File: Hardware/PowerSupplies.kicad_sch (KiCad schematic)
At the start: 56 parts

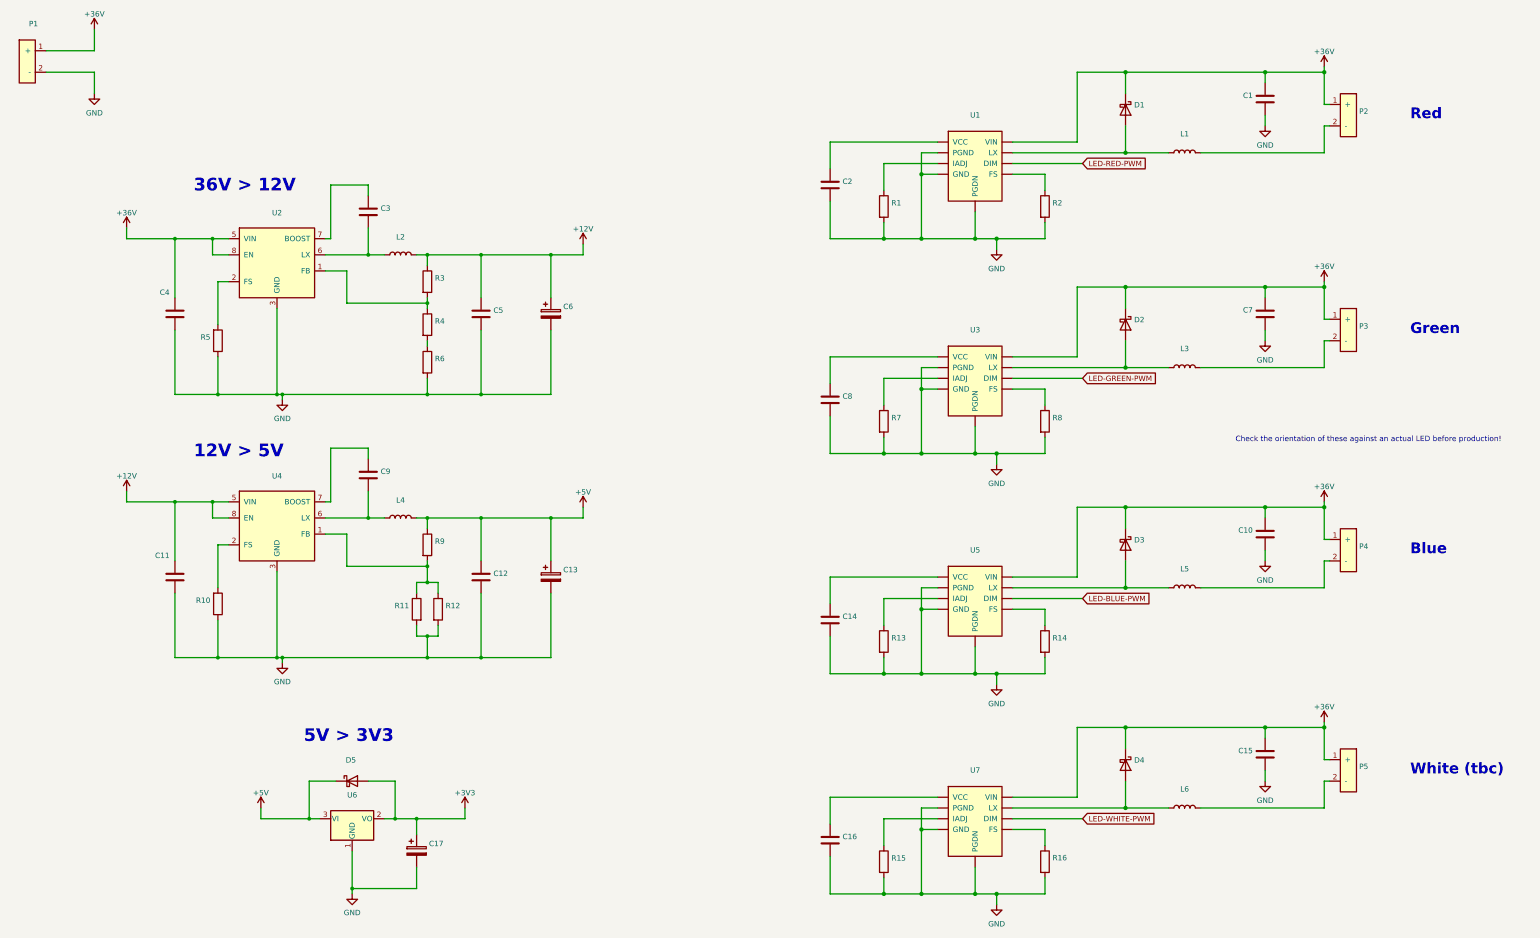
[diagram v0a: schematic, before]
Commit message: Xtal footprint selected. Remaining parts need new footprints.
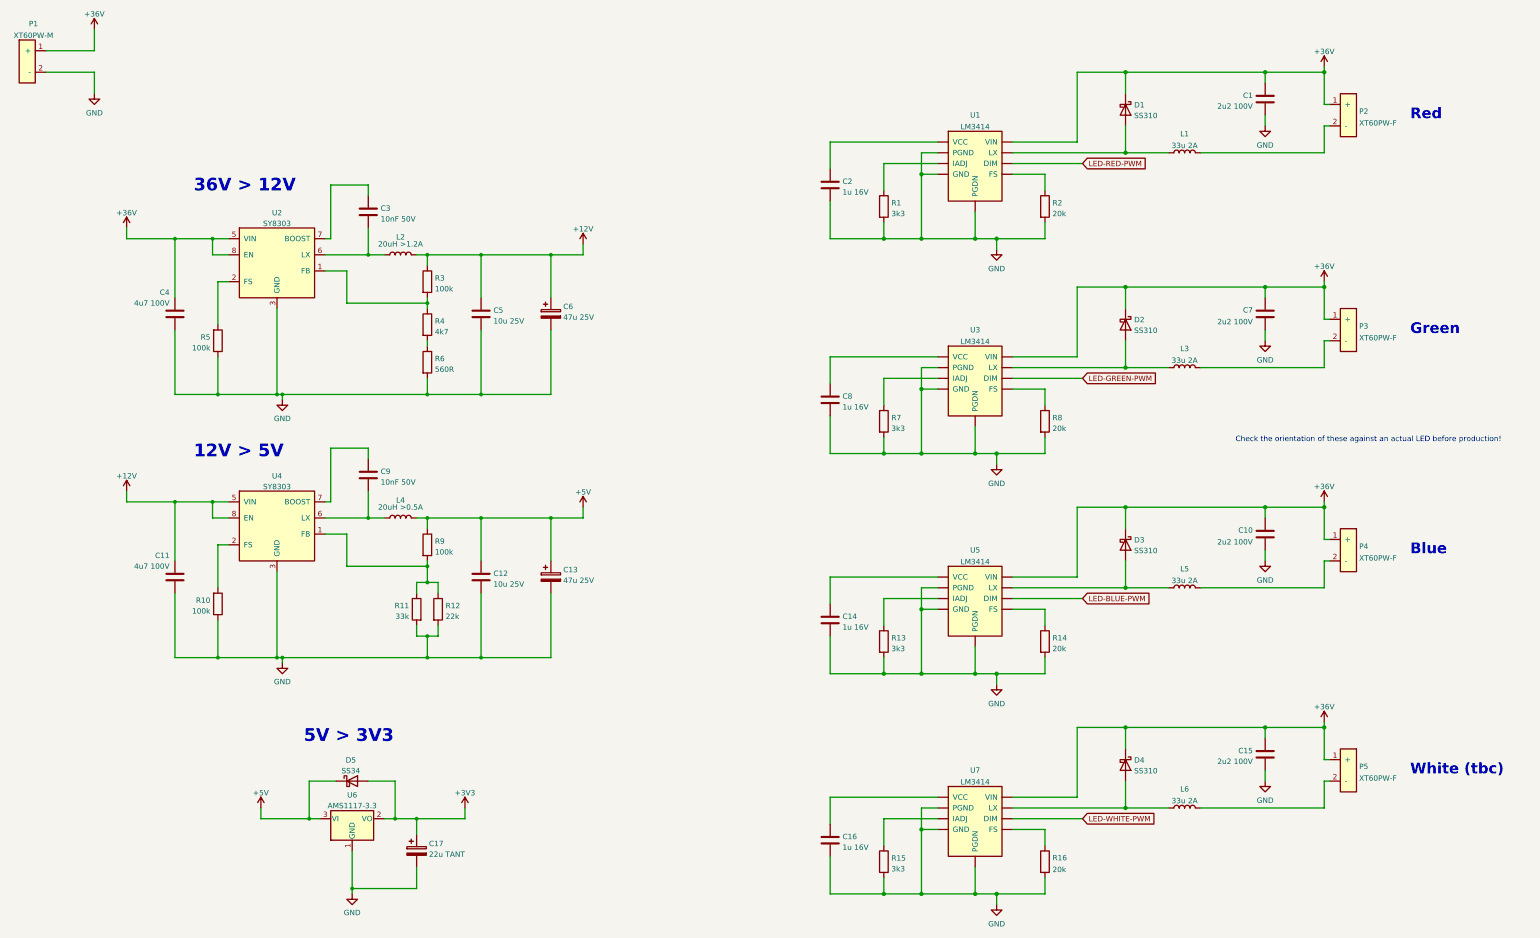
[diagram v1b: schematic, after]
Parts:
- C1, C10, C15, C7: value (none) -> 2u2 100V; footprint (none) -> Capacitor_SMD:CP_Elec_6.3x5.4
- C11, C4: value (none) -> 4u7 100V; footprint (none) -> Capacitor_SMD:C_1210_3225Metric
- C12, C5: value (none) -> 10u 25V; footprint (none) -> Capacitor_SMD:C_0805_2012Metric_Pad1.18x1.45mm_HandSolder
- C13, C6: value (none) -> 47u 25V; footprint (none) -> Capacitor_SMD:CP_Elec_6.3x5.4
- C14, C16, C2, C8: value (none) -> 1u 16V; footprint (none) -> Capacitor_SMD:C_0805_2012Metric_Pad1.18x1.45mm_HandSolder
- C17: value (none) -> 22u TANT; footprint (none) -> Capacitor_Tantalum_SMD:CP_EIA-3528-15_AVX-H
- C3, C9: value (none) -> 10nF 50V; footprint (none) -> Capacitor_SMD:C_0805_2012Metric_Pad1.18x1.45mm_HandSolder
- D1, D2, D3, D4: value (none) -> SS310; footprint (none) -> Diode_SMD:D_SMA_Handsoldering
- D5: value (none) -> SS34; footprint (none) -> Diode_SMD:D_SMA_Handsoldering
- L1, L3, L5, L6: value (none) -> 33u 2A; footprint (none) -> Inductor_SMD:L_SigTra_SC3316F
- L2: value (none) -> 20uH >1.2A; footprint (none) -> Inductor_SMD:L_Taiyo-Yuden_NR-80xx
- L4: value (none) -> 20uH >0.5A; footprint (none) -> Inductor_SMD:L_Taiyo-Yuden_NR-80xx
- P1: value (none) -> XT60PW-M; footprint (none) -> PersonalConnectors:AMASS_XT60PW-M
- P2, P3, P4, P5: value (none) -> XT60PW-F; footprint (none) -> PersonalConnectors:AMASS_XT60PW-F
- R1, R13, R15, R7: value (none) -> 3k3; footprint (none) -> Resistor_SMD:R_0603_1608Metric_Pad0.98x0.95mm_HandSolder
- R10, R3, R5, R9: value (none) -> 100k; footprint (none) -> Resistor_SMD:R_0603_1608Metric_Pad0.98x0.95mm_HandSolder
- R11: value (none) -> 33k; footprint (none) -> Resistor_SMD:R_0603_1608Metric_Pad0.98x0.95mm_HandSolder
- R12: value (none) -> 22k; footprint (none) -> Resistor_SMD:R_0603_1608Metric_Pad0.98x0.95mm_HandSolder
- R14, R16, R2, R8: value (none) -> 20k; footprint (none) -> Resistor_SMD:R_0603_1608Metric_Pad0.98x0.95mm_HandSolder
- R4: value (none) -> 4k7; footprint (none) -> Resistor_SMD:R_0603_1608Metric_Pad0.98x0.95mm_HandSolder
- R6: value (none) -> 560R; footprint (none) -> Resistor_SMD:R_0603_1608Metric_Pad0.98x0.95mm_HandSolder
- U1, U3, U5, U7: value (none) -> LM3414; footprint (none) -> PersonalDiscretes:TI_SO-PowerPAD-8_HandSolder
- U2, U4: value (none) -> SY8303; footprint (none) -> Package_TO_SOT_SMD:TSOT-23-8
- U6: value (none) -> AMS1117-3.3; footprint (none) -> Package_TO_SOT_SMD:SOT-223-3_TabPin2

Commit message: USB footprint added, mount holes added.
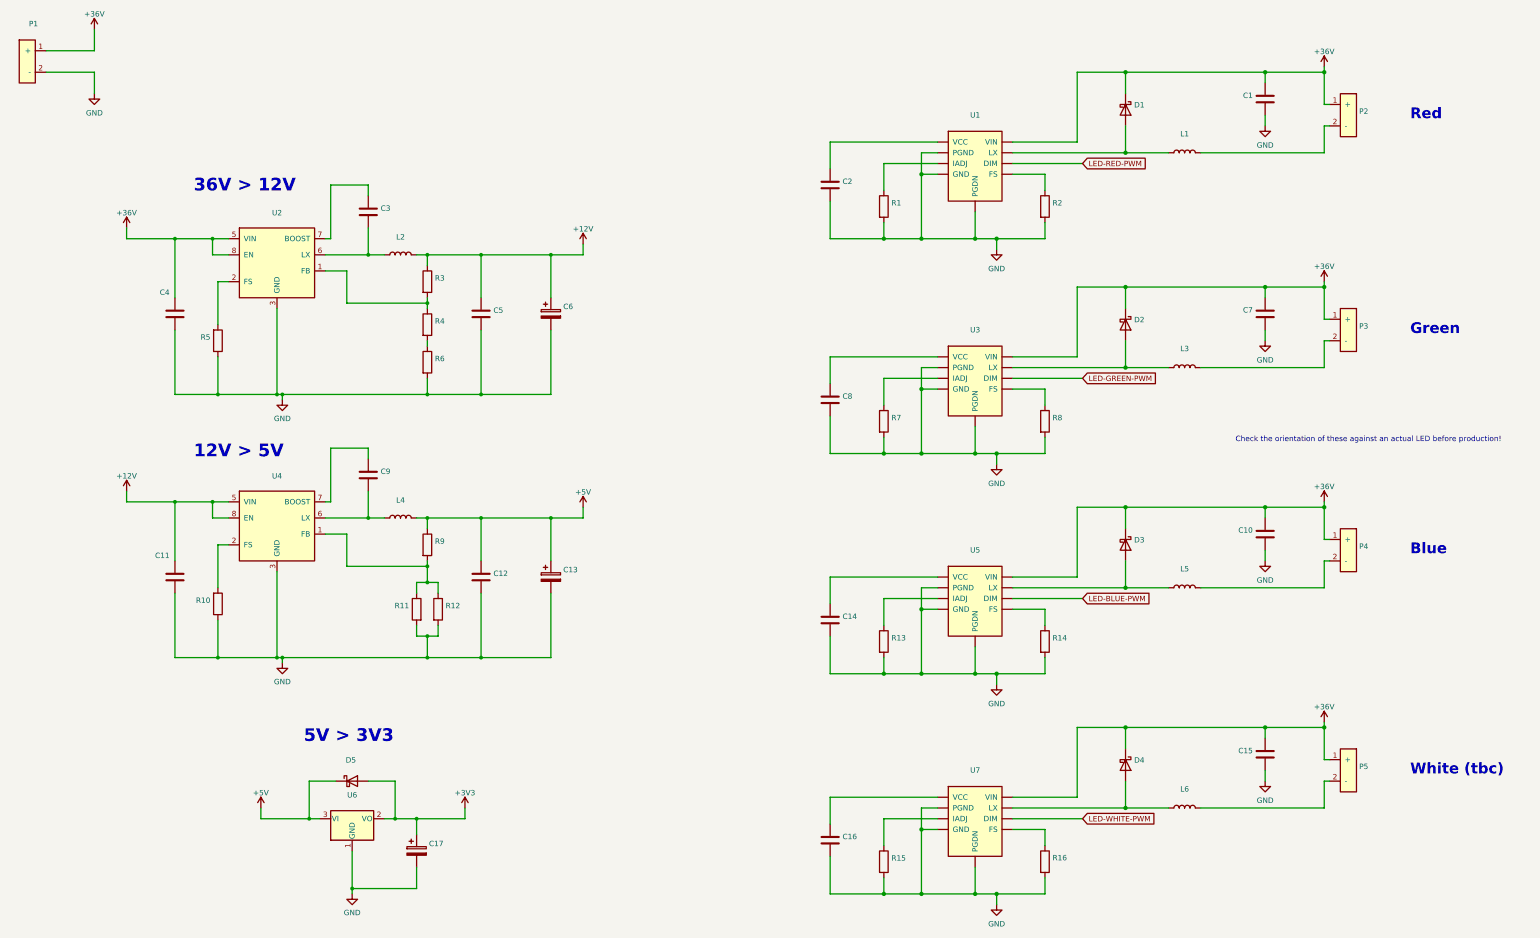
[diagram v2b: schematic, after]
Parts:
- C1, C10, C15, C7: value 2u2 100V -> (none); footprint Capacitor_SMD:CP_Elec_6.3x5.4 -> (none)
- C11, C4: value 4u7 100V -> (none); footprint Capacitor_SMD:C_1210_3225Metric -> (none)
- C12, C5: value 10u 25V -> (none); footprint Capacitor_SMD:C_0805_2012Metric_Pad1.18x1.45mm_HandSolder -> (none)
- C13, C6: value 47u 25V -> (none); footprint Capacitor_SMD:CP_Elec_6.3x5.4 -> (none)
- C14, C16, C2, C8: value 1u 16V -> (none); footprint Capacitor_SMD:C_0805_2012Metric_Pad1.18x1.45mm_HandSolder -> (none)
- C17: value 22u TANT -> (none); footprint Capacitor_Tantalum_SMD:CP_EIA-3528-15_AVX-H -> (none)
- C3, C9: value 10nF 50V -> (none); footprint Capacitor_SMD:C_0805_2012Metric_Pad1.18x1.45mm_HandSolder -> (none)
- D1, D2, D3, D4: value SS310 -> (none); footprint Diode_SMD:D_SMA_Handsoldering -> (none)
- D5: value SS34 -> (none); footprint Diode_SMD:D_SMA_Handsoldering -> (none)
- L1, L3, L5, L6: value 33u 2A -> (none); footprint Inductor_SMD:L_SigTra_SC3316F -> (none)
- L2: value 20uH >1.2A -> (none); footprint Inductor_SMD:L_Taiyo-Yuden_NR-80xx -> (none)
- L4: value 20uH >0.5A -> (none); footprint Inductor_SMD:L_Taiyo-Yuden_NR-80xx -> (none)
- P1: value XT60PW-M -> (none); footprint PersonalConnectors:AMASS_XT60PW-M -> (none)
- P2, P3, P4, P5: value XT60PW-F -> (none); footprint PersonalConnectors:AMASS_XT60PW-F -> (none)
- R1, R13, R15, R7: value 3k3 -> (none); footprint Resistor_SMD:R_0603_1608Metric_Pad0.98x0.95mm_HandSolder -> (none)
- R10, R3, R5, R9: value 100k -> (none); footprint Resistor_SMD:R_0603_1608Metric_Pad0.98x0.95mm_HandSolder -> (none)
- R11: value 33k -> (none); footprint Resistor_SMD:R_0603_1608Metric_Pad0.98x0.95mm_HandSolder -> (none)
- R12: value 22k -> (none); footprint Resistor_SMD:R_0603_1608Metric_Pad0.98x0.95mm_HandSolder -> (none)
- R14, R16, R2, R8: value 20k -> (none); footprint Resistor_SMD:R_0603_1608Metric_Pad0.98x0.95mm_HandSolder -> (none)
- R4: value 4k7 -> (none); footprint Resistor_SMD:R_0603_1608Metric_Pad0.98x0.95mm_HandSolder -> (none)
- R6: value 560R -> (none); footprint Resistor_SMD:R_0603_1608Metric_Pad0.98x0.95mm_HandSolder -> (none)
- U1, U3, U5, U7: value LM3414 -> (none); footprint PersonalDiscretes:TI_SO-PowerPAD-8_HandSolder -> (none)
- U2, U4: value SY8303 -> (none); footprint Package_TO_SOT_SMD:TSOT-23-8 -> (none)
- U6: value AMS1117-3.3 -> (none); footprint Package_TO_SOT_SMD:SOT-223-3_TabPin2 -> (none)
